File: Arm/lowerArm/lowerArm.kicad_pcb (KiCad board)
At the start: 2 copper layers, 58.7 x 70.8 mm, 5 parts, among them J1 Screw_Terminal_01x12, J2 Screw_Terminal_01x12, U1 LM1084-5.0

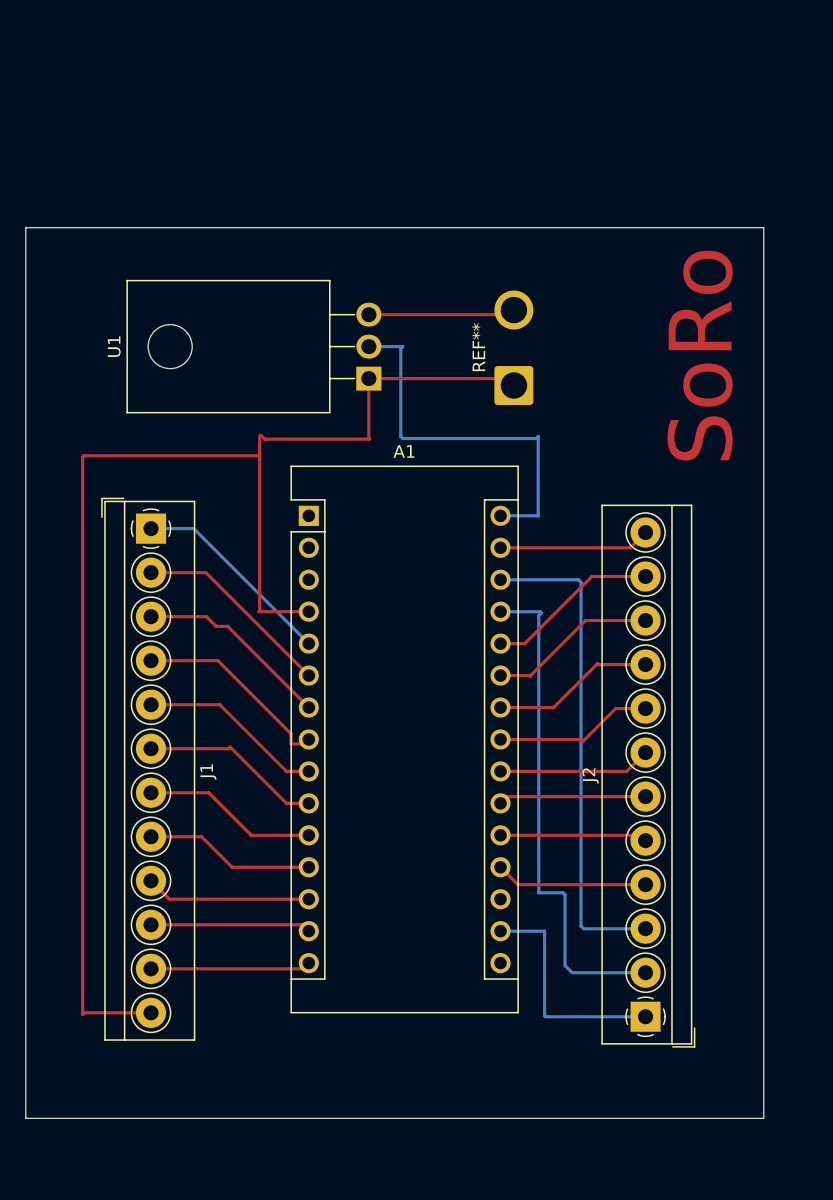
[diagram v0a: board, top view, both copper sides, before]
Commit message: updated Arm arduino code, manual_operate, and PCBs
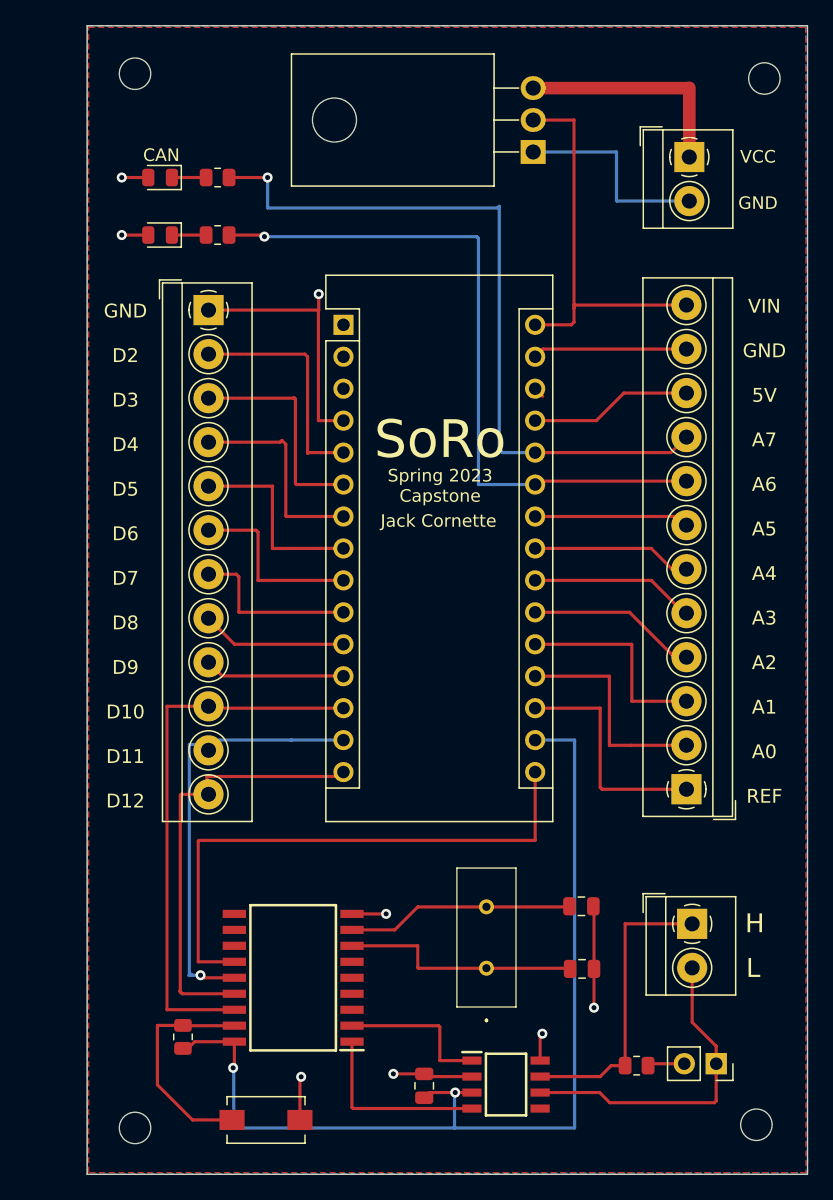
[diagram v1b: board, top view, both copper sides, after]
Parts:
- removed the REF** at (152.0, 73.1)
- added C1: 0.1uF, Capacitor_SMD:C_0805_2012Metric, F.Cu at (144.9, 128.7)
- added C2: 22pF, Capacitor_SMD:C_0805_2012Metric, F.Cu at (157.5, 119.4)
- added C3: 22pF, Capacitor_SMD:C_0805_2012Metric, F.Cu at (157.4, 114.5)
- added CAN: LED_0805_2012Metric, LED_SMD:LED_0805_2012Metric, F.Cu at (123.9, 56.5)
- added J3: Screw_Terminal_01x02, TerminalBlock_4Ucon:TerminalBlock_4Ucon_1x02_P3.50mm_Horizontal, F.Cu at (166.0, 54.9)
- added J3: Screw_Terminal_01x02, TerminalBlock_4Ucon:TerminalBlock_4Ucon_1x02_P3.50mm_Horizontal, F.Cu at (166.2, 115.9)
- added R2: 10k, Resistor_SMD:R_0805_2012Metric, F.Cu at (125.7, 124.8)
- added R3: R_US, Resistor_SMD:R_0805_2012Metric, F.Cu at (128.5, 61.1)
- added R3: R_US, Resistor_SMD:R_0805_2012Metric, F.Cu at (161.8, 127.1)
- added R3: R_US, Resistor_SMD:R_0805_2012Metric, F.Cu at (128.5, 56.5)
- added REF**: SW_SPST_EVQPE1, Button_Switch_SMD:SW_SPST_EVQPE1, F.Cu at (132.3, 131.4)
- added REF**: MountingHole_2.5mm, MountingHole:MountingHole_2.5mm, F.Cu at (172.0, 48.6)
- added REF**: PinSocket_1x02_P2.54mm_Vertical, Connector_PinSocket_2.54mm:PinSocket_1x02_P2.54mm_Vertical, F.Cu at (168.1, 127.0)
- added REF**: MountingHole_2.5mm, MountingHole:MountingHole_2.5mm, F.Cu at (171.3, 131.8)
- added REF**: MountingHole_2.5mm, MountingHole:MountingHole_2.5mm, F.Cu at (121.9, 48.3)
- added REF**: LED_0805_2012Metric, LED_SMD:LED_0805_2012Metric, F.Cu at (123.9, 61.1)
- added REF**: MountingHole_2.5mm, MountingHole:MountingHole_2.5mm, F.Cu at (121.9, 132.1)
- added U2: Crystal_Oscillator_8MHz, LFXTAL:LFXTAL057135Bulk, F.Cu at (149.9, 119.4)
- added U3: MCP2515-xSO, MCP2515_SMD:SOIC127P1030X265-18N, F.Cu at (134.5, 120.1)
- added U4: MAX3051, MAX3051:SOIC127P600X175-8N, F.Cu at (151.4, 128.6)
- moved U1 22.3 mm to (153.6, 54.5)
- moved J2 18.4 mm to (165.8, 105.2)
- moved J1 18.0 mm to (127.8, 67.1)
- moved A1 15.4 mm to (138.5, 68.2)
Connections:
- A1 pad 16: unconnected-(A1-Pad16) -> Net-(A1-Pad16)
- A1 pad 5: Net-(A1-Pad5) -> unconnected-(A1-Pad5)
- J1 pad 1: Net-(A1-Pad5) -> GND
- J1 pad 10: Net-(A1-Pad14) -> Net-(A1-Pad13)
- J1 pad 11: Net-(A1-Pad15) -> Net-(A1-Pad14)
- J1 pad 12: GND -> Net-(A1-Pad15)
- J1 pad 2: Net-(A1-Pad6) -> unconnected-(A1-Pad5)
- J1 pad 3: Net-(A1-Pad7) -> Net-(A1-Pad6)
- J1 pad 4: Net-(A1-Pad8) -> Net-(A1-Pad7)
- J1 pad 5: Net-(A1-Pad9) -> Net-(A1-Pad8)
- J1 pad 6: Net-(A1-Pad10) -> Net-(A1-Pad9)
- J1 pad 7: Net-(A1-Pad11) -> Net-(A1-Pad10)
- J1 pad 8: Net-(A1-Pad12) -> Net-(A1-Pad11)
- J1 pad 9: Net-(A1-Pad13) -> Net-(A1-Pad12)
- J2 pad 1: Net-(A1-Pad17) -> unconnected-(A1-Pad18)
- J2 pad 10: Net-(A1-Pad25) -> Net-(A1-Pad27)
- J2 pad 11: Net-(A1-Pad26) -> Net-(A1-Pad29)
- J2 pad 12: Net-(A1-Pad29) -> Net-(A1-Pad30)
- J2 pad 2: Net-(A1-Pad27) -> Net-(A1-Pad19)
- J2 pad 3: Net-(A1-Pad28) -> Net-(A1-Pad20)
- J2 pad 4: Net-(A1-Pad19) -> Net-(A1-Pad21)
- J2 pad 5: Net-(A1-Pad20) -> Net-(A1-Pad22)
- J2 pad 6: Net-(A1-Pad21) -> Net-(A1-Pad23)
- J2 pad 7: Net-(A1-Pad22) -> Net-(A1-Pad24)
- J2 pad 8: Net-(A1-Pad23) -> Net-(A1-Pad25)
- J2 pad 9: Net-(A1-Pad24) -> Net-(A1-Pad26)
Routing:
- net Net-(A1-Pad17): track 18.3 -> 78.9 mm, vias 0 -> 2
- net Net-(A1-Pad26): track 13.7 -> 58.8 mm, vias 0 -> 1
- net Net-(A1-Pad16): track 0.00 -> 44.7 mm
- net GND: track 107.3 -> 64.2 mm, vias 0 -> 8
- net Net-(A1-Pad25): track 13.4 -> 56.3 mm, vias 0 -> 1
- net Net-(A1-Pad28): track 39.0 -> 0.85 mm
- net Net-(A1-Pad13): track 13.2 -> 43.8 mm
- net Net-(A1-Pad27): track 40.0 -> 12.9 mm
- net Net-(J3-Pad2): track 0.00 -> 25.8 mm
- net Net-(J3-Pad1): track 0.00 -> 23.7 mm
- net Net-(A1-Pad14): track 12.8 -> 35.5 mm, vias 0 -> 1
- net Net-(A1-Pad15): track 12.7 -> 34.9 mm
- net Net-(C2-Pad1): track 0.00 -> 19.1 mm
- net unconnected-(A1-Pad5): track 0.00 -> 18.5 mm
- net unconnected-(A1-Pad18): track 0.00 -> 18.4 mm
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- added copper zone on B.Cu, net GND
- added copper zone on F.Cu, net Net-(A1-Pad30)
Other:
- board size 58.7 x 70.8 mm -> 57.3 x 91.3 mm
- board text added: "GND"
- board text added: "GND D2 D3 D4 D5 D6 D7 D8 D9 D10 D11 D12"
- board text added: "H"
- board text added: "Jack Cornette"
- board text added: "L"
- board text added: "Spring 2023 Capstone"
- board text added: "VCC"
- board text added: "VIN GND 5V A7 A6 A5 A4 A3 A2 A1 A0 REF"
